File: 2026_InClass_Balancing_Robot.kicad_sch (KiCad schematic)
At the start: 52 parts, among them J1 M2_CONN, J2 M1_CONN, J3 BAT_CONN, J4 CONN_MPU6050, J5 MT6701_CONN, J6 ENCODER_CONN, J7 Conn_01x04, J8 USB_C_Receptacle, SW1 SW_uP_Reset, U1 STM32F401RBTx, U2 LD1117S50TR_SOT223, U3 LD1117S50TR_SOT223, U4 TB6612FNG, U5 ESP8266-01_ESP-01, U6 USBLC6-2SC6

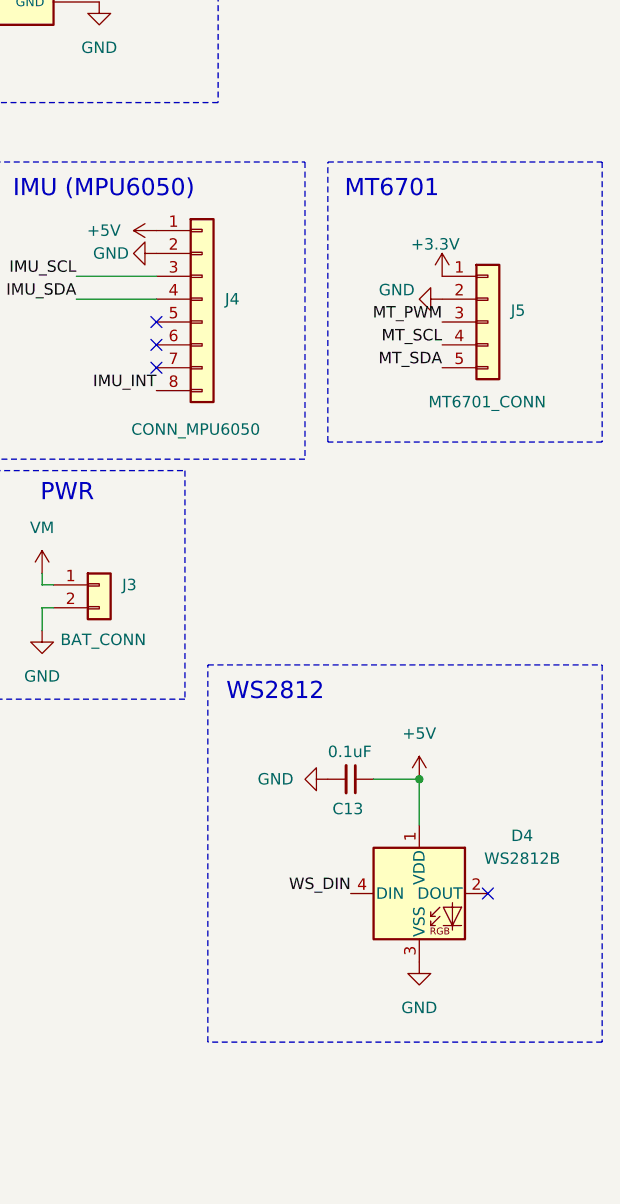
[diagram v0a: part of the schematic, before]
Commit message: all files in project
layout from class
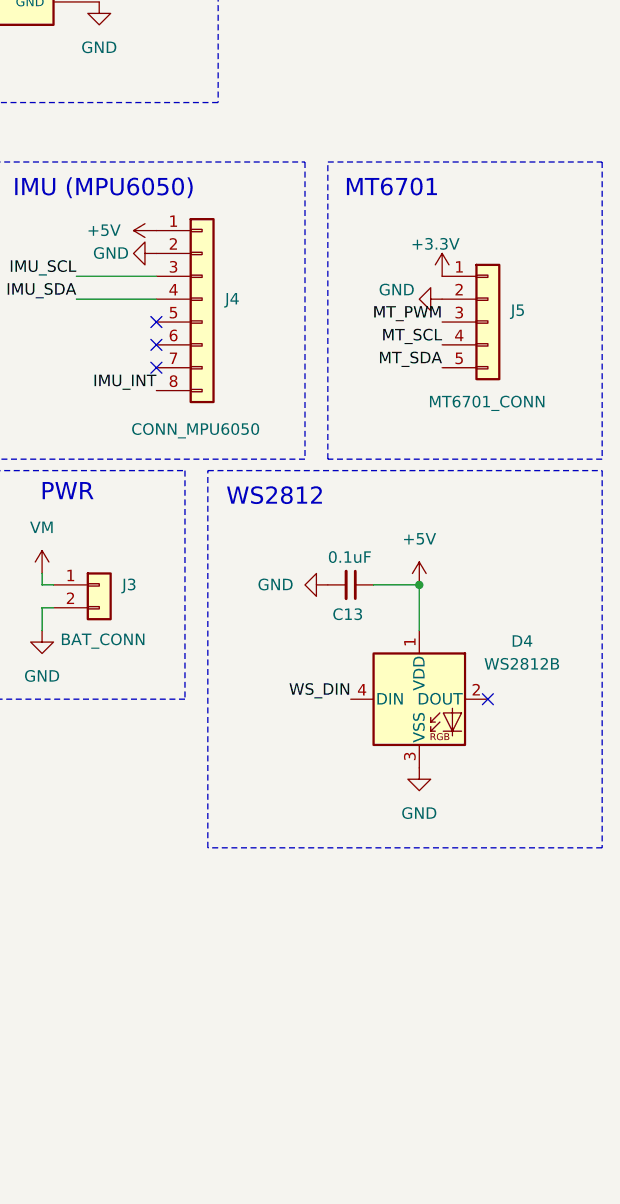
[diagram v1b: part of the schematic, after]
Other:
- moved on the sheet: C13, D4
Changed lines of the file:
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@@
 	(rectangle
 		(start 248.92 59.69)
-		(end 279.4 90.805)
+		(end 279.4 92.71)
 		(stroke
 			(width 0)
@@
 	)
 	(rectangle
-		(start 235.585 115.57)
-		(end 279.4 157.48)
+		(start 235.585 93.98)
+		(end 279.4 135.89)
 		(stroke
 			(width 0)
@@
 	(text "WS2812"
 		(exclude_from_sim no)
-		(at 243.078 118.618 0)
+		(at 243.078 97.028 0)
 		(effects
 			(font
@@
 	)
 	(junction
-		(at 259.08 128.27)
+		(at 259.08 106.68)
 		(diameter 0)
 		(color 0 0 0 0)
@@
 	)
 	(no_connect
-		(at 266.7 140.97)
+		(at 266.7 119.38)
 	)
 	(no_connect
@@
 	(wire
 		(pts
-			(xy 259.08 128.27) (xy 259.08 133.35)
+			(xy 259.08 106.68) (xy 259.08 111.76)
 		)
 		(stroke
@@
 	(wire
 		(pts
-			(xy 254 128.27) (xy 259.08 128.27)
+			(xy 254 106.68) (xy 259.08 106.68)
 		)
 		(stroke
@@
 	)
 	(label "WS_DIN"
-		(at 251.46 140.97 180)
+		(at 251.46 119.38 180)
 		(effects
 			(font
@@
 	(symbol
 		(lib_id "power:GND")
-		(at 259.08 148.59 0)
+		(at 259.08 127 0)
 		(unit 1)
 		(exclude_from_sim no)
@@
 		(fields_autoplaced yes)
 		(property "Reference" "#PWR033"
-			(at 259.08 154.94 0)
+			(at 259.08 133.35 0)
 			(effects
 				(font
@@
 		)
 		(property "Value" "GND"
-			(at 259.08 153.67 0)
+			(at 259.08 132.08 0)
 			(effects
 				(font
@@
 		)
 		(property "Footprint" ""
-			(at 259.08 148.59 0)
+			(at 259.08 127 0)
 			(effects
 				(font
@@
 		)
 		(property "Datasheet" ""
-			(at 259.08 148.59 0)
+			(at 259.08 127 0)
 			(effects
 				(font
@@
 		)
 		(property "Description" "Power symbol creates a global label with name \"GND\" , ground"
-			(at 259.08 148.59 0)
+			(at 259.08 127 0)
 			(effects
 				(font
@@
 	(symbol
 		(lib_id "LED:WS2812B")
-		(at 259.08 140.97 0)
+		(at 259.08 119.38 0)
 		(unit 1)
 		(exclude_from_sim no)
@@
 		(fields_autoplaced yes)
 		(property "Reference" "D4"
-			(at 270.51 134.5498 0)
+			(at 270.51 112.9598 0)
 			(effects
 				(font
@@
 		)
 		(property "Value" "WS2812B"
-			(at 270.51 137.0898 0)
+			(at 270.51 115.4998 0)
 			(effects
 				(font
@@
 		)
 		(property "Footprint" "LED_SMD:LED_WS2812B_PLCC4_5.0x5.0mm_P3.2mm"
-			(at 260.35 148.59 0)
+			(at 260.35 127 0)
 			(effects
 				(font
@@
 		)
 		(property "Datasheet" "https://cdn-shop.adafruit.com/datasheets/WS2812B.pdf"
-			(at 261.62 150.495 0)
+			(at 261.62 128.905 0)
 			(effects
 				(font
@@
 		)
 		(property "Description" "RGB LED with integrated controller"
-			(at 259.08 140.97 0)
+			(at 259.08 119.38 0)
 			(effects
 				(font
@@
 	(symbol
 		(lib_id "Device:C_Small")
-		(at 251.46 128.27 270)
+		(at 251.46 106.68 270)
 		(unit 1)
 		(exclude_from_sim no)
@@
 		(dnp no)
 		(property "Reference" "C13"
-			(at 249.428 131.572 90)
+			(at 249.428 109.982 90)
 			(effects
 				(font
@@
 		)
 		(property "Value" "0.1uF"
-			(at 248.92 125.222 90)
+			(at 248.92 103.632 90)
 			(effects
 				(font
@@
 		)
 		(property "Footprint" "Capacitor_SMD:C_0805_2012Metric_Pad1.18x1.45mm_HandSolder"
-			(at 251.46 128.27 0)
+			(at 251.46 106.68 0)
 			(effects
 				(font
@@
 		)
 		(property "Datasheet" "~"
-			(at 251.46 128.27 0)
+			(at 251.46 106.68 0)
 			(effects
 				(font
@@
 		)
 		(property "Description" "Unpolarized capacitor, small symbol"
-			(at 251.46 128.27 0)
+			(at 251.46 106.68 0)
 			(effects
 				(font
@@
 		)
 		(property "Mouser" "https://www.mouser.com/ProductDetail/KYOCERA-AVX/KAM21BR71H104JM?qs=Jm2GQyTW%2FbjKdz3nqUKYQg%3D%3D"
-			(at 251.46 128.27 0)
+			(at 251.46 106.68 0)
 			(effects
 				(font
@@
 		)
 		(property "Unit Price" "0.20"
-			(at 251.46 128.27 0)
+			(at 251.46 106.68 0)
 			(effects
 				(font
@@
 		)
 		(property "Mfr. #" "KAM21BR71H104JM"
-			(at 251.46 128.27 0)
+			(at 251.46 106.68 0)
 			(effects
 				(font
@@
 	(symbol
 		(lib_id "power:GND")
-		(at 248.92 128.27 270)
+		(at 248.92 106.68 270)
 		(unit 1)
 		(exclude_from_sim no)
@@
 		(fields_autoplaced yes)
 		(property "Reference" "#PWR031"
-			(at 242.57 128.27 0)
+			(at 242.57 106.68 0)
 			(effects
 				(font
@@
 		)
 		(property "Value" "GND"
-			(at 245.11 128.2699 90)
+			(at 245.11 106.6799 90)
 			(effects
 				(font
@@
 		)
 		(property "Footprint" ""
-			(at 248.92 128.27 0)
+			(at 248.92 106.68 0)
 			(effects
 				(font
@@
 		)
 		(property "Datasheet" ""
-			(at 248.92 128.27 0)
+			(at 248.92 106.68 0)
 			(effects
 				(font
@@
 		)
 		(property "Description" "Power symbol creates a global label with name \"GND\" , ground"
-			(at 248.92 128.27 0)
+			(at 248.92 106.68 0)
 			(effects
 				(font
@@
 	(symbol
 		(lib_id "power:+3.3V")
-		(at 259.08 128.27 0)
+		(at 259.08 106.68 0)
 		(unit 1)
 		(exclude_from_sim no)
@@
 		(fields_autoplaced yes)
 		(property "Reference" "#PWR032"
-			(at 259.08 132.08 0)
+			(at 259.08 110.49 0)
 			(effects
 				(font
@@
 		)
 		(property "Value" "+5V"
-			(at 259.08 123.19 0)
+			(at 259.08 101.6 0)
 			(effects
 				(font
@@
 		)
 		(property "Footprint" ""
-			(at 259.08 128.27 0)
+			(at 259.08 106.68 0)
 			(effects
 				(font
@@
 		)
 		(property "Datasheet" ""
-			(at 259.08 128.27 0)
+			(at 259.08 106.68 0)
 			(effects
 				(font
@@
 		)
 		(property "Description" "Power symbol creates a global label with name \"+3.3V\""
-			(at 259.08 128.27 0)
+			(at 259.08 106.68 0)
 			(effects
 				(font
